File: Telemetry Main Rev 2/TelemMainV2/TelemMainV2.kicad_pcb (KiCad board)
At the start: 2 copper layers, 161 x 113.3 mm, 59 parts, among them J1 8 pin ATM connector, J2 40 pin ZIF FPC Connector, J3 12 pin ATM connector, J4 SD to SPI (Molex nanofit), U1 LM7805_TO220, U2 LM7809_TO220, U3 NUCLEO-F446RE, U4 ISO1050DUB, U5 XBP9B-DPST-001, U6 MCP6004, U7 BT817Q, U8 ISO1050DUB

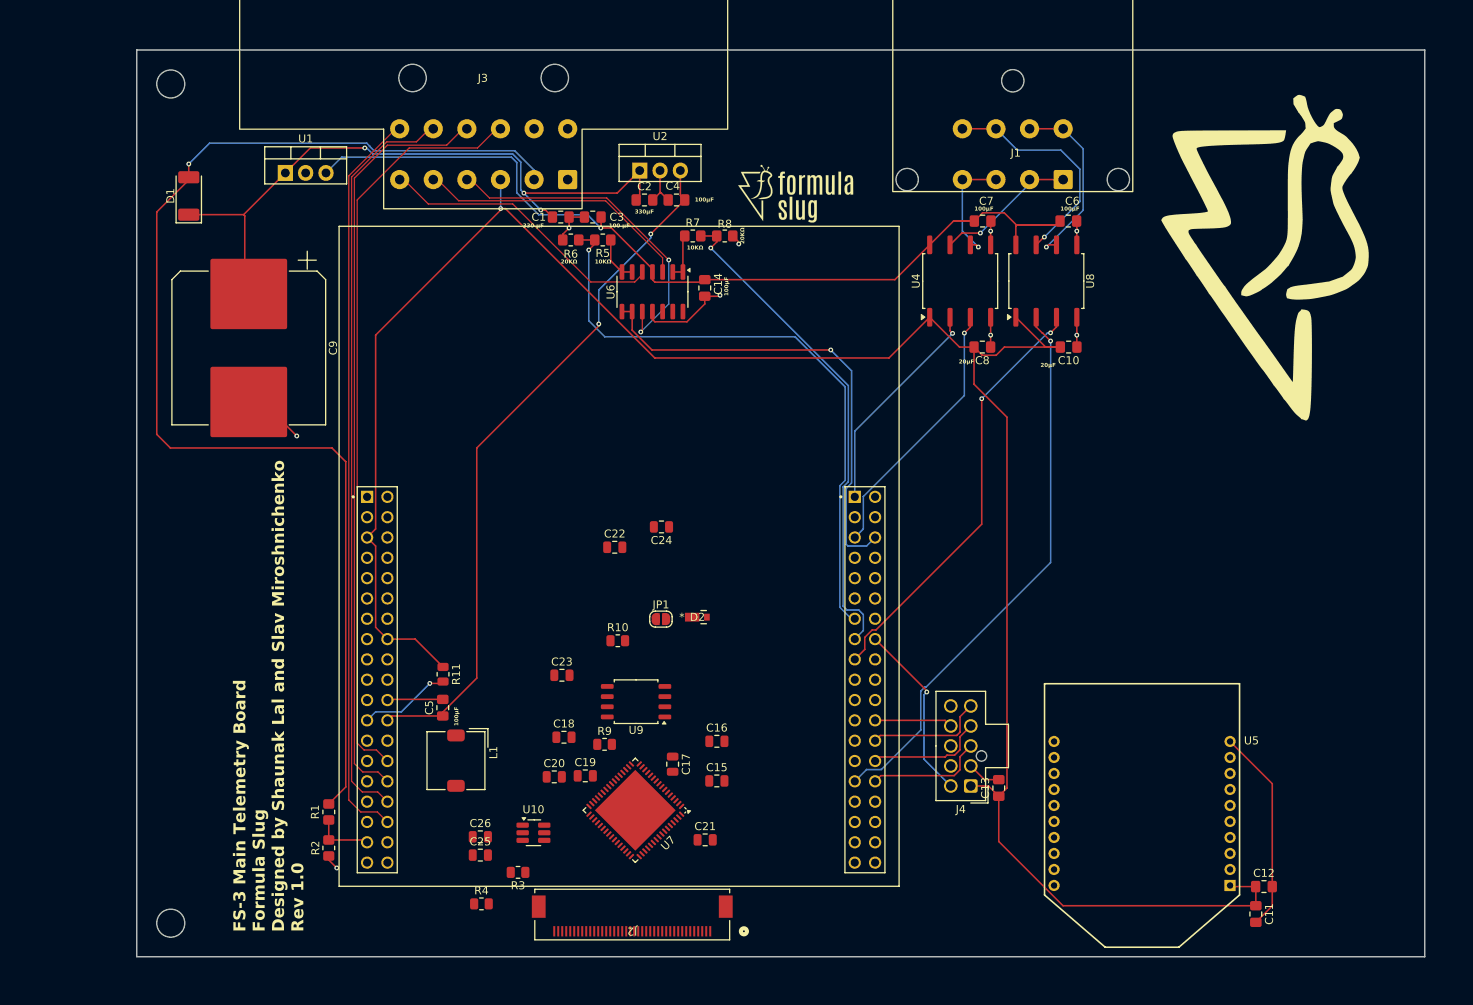
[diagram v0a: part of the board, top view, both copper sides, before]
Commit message: dash traces
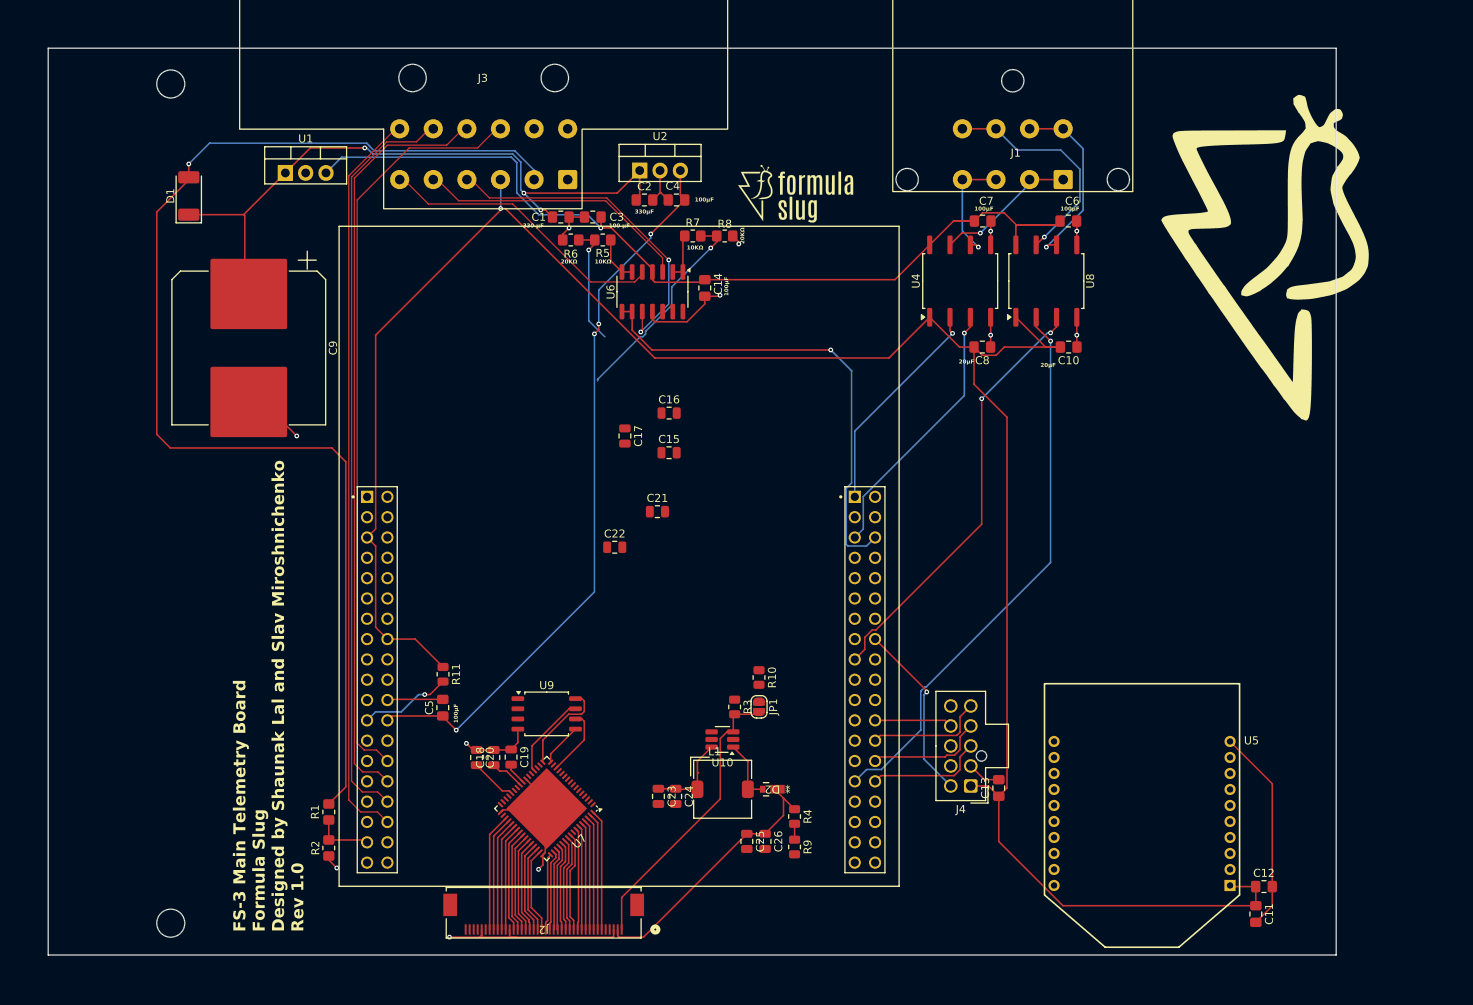
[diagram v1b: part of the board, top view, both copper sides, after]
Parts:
- moved C15 41.5 mm to (133.5, 93.6)
- moved C16 41.5 mm to (133.5, 88.6)
- moved C21 41.5 mm to (132.1, 101.0)
- moved C17 41.5 mm to (128.0, 91.5)
- moved R4 40.6 mm to (149.2, 139.1), turned to -90 degrees
- moved C26 35.6 mm to (145.5, 142.2), turned to -90 degrees
- moved R3 34.1 mm to (141.7, 125.4), turned to -90 degrees
- moved C24 33.7 mm to (134.4, 136.5), turned to -90 degrees
- moved L1 33.5 mm to (140.2, 135.7), turned to 0 degrees
- moved C25 33.4 mm to (143.3, 142.2), turned to -90 degrees
- moved R9 27.0 mm to (149.2, 142.9), turned to -90 degrees
- moved U10 26.3 mm to (140.2, 129.4), turned to 180 degrees
- moved D2 23.5 mm to (146.4, 135.7), turned to 180 degrees
- moved C23 19.4 mm to (132.2, 136.5), turned to -90 degrees
- moved R10 18.2 mm to (144.8, 121.7), turned to -90 degrees
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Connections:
- U3 pad CN10_12: Radio RTS1 -> unconnected-(U3B-PA12-PadCN10_12)
- U3 pad CN10_14: Radio CTS1 -> unconnected-(U3B-PA11-PadCN10_14)
- U3 pad CN10_21: Radio TX1 -> unconnected-(U3B-PA9-PadCN10_21)
- U3 pad CN10_33: Radio RX1 -> unconnected-(U3B-PA10-PadCN10_33)
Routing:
- net Brake Sensor R 3V3: track 78.2 -> 15.2 mm
- net GND: track 83.7 -> 135.1 mm, vias 9 -> 12
- net BL-Low: track 0.00 -> 36.4 mm
- net Brake Sensor F 3V3: track 62.4 -> 26.5 mm
- net BL-High: track 0.00 -> 33.4 mm
- net +3V3: track 272.7 -> 293.3 mm
- net R1: track 0.00 -> 15.1 mm
- net DEN: track 0.00 -> 14.8 mm
- net R2: track 0.00 -> 14.7 mm
- net VSYNC: track 0.00 -> 14.4 mm
- net R3: track 0.00 -> 14.3 mm
- net HSYNC: track 0.00 -> 14.0 mm
- net R4: track 0.00 -> 13.8 mm
- net DISP: track 0.00 -> 13.5 mm
- net R5: track 0.00 -> 13.4 mm
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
